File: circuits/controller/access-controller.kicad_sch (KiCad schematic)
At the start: 64 parts, among them J1 Conn_01x01_Female, J10 Terminal_01x03, J11 Terminal_01x04, J12 Screw_Terminal_01x05, J13 Conn_02x06_Odd_Even, J14 Terminal_01x04, J15 Terminal_01x03, J16 Terminal_01x03, J17 Terminal_01x03, J18 Terminal_01x04, J19 Screw_Terminal_01x05, J2 Conn_01x01_Female, J3 Conn_01x01_Female, J4 Conn_01x01_Female, J6 Screw_Terminal_01x02, J7 Terminal_01x04, J8 Terminal_01x03, J9 Barrel_Jack_Switch, J9 Terminal_01x03, Q3 Q_MMBT5551, U1 MCP23017_SS

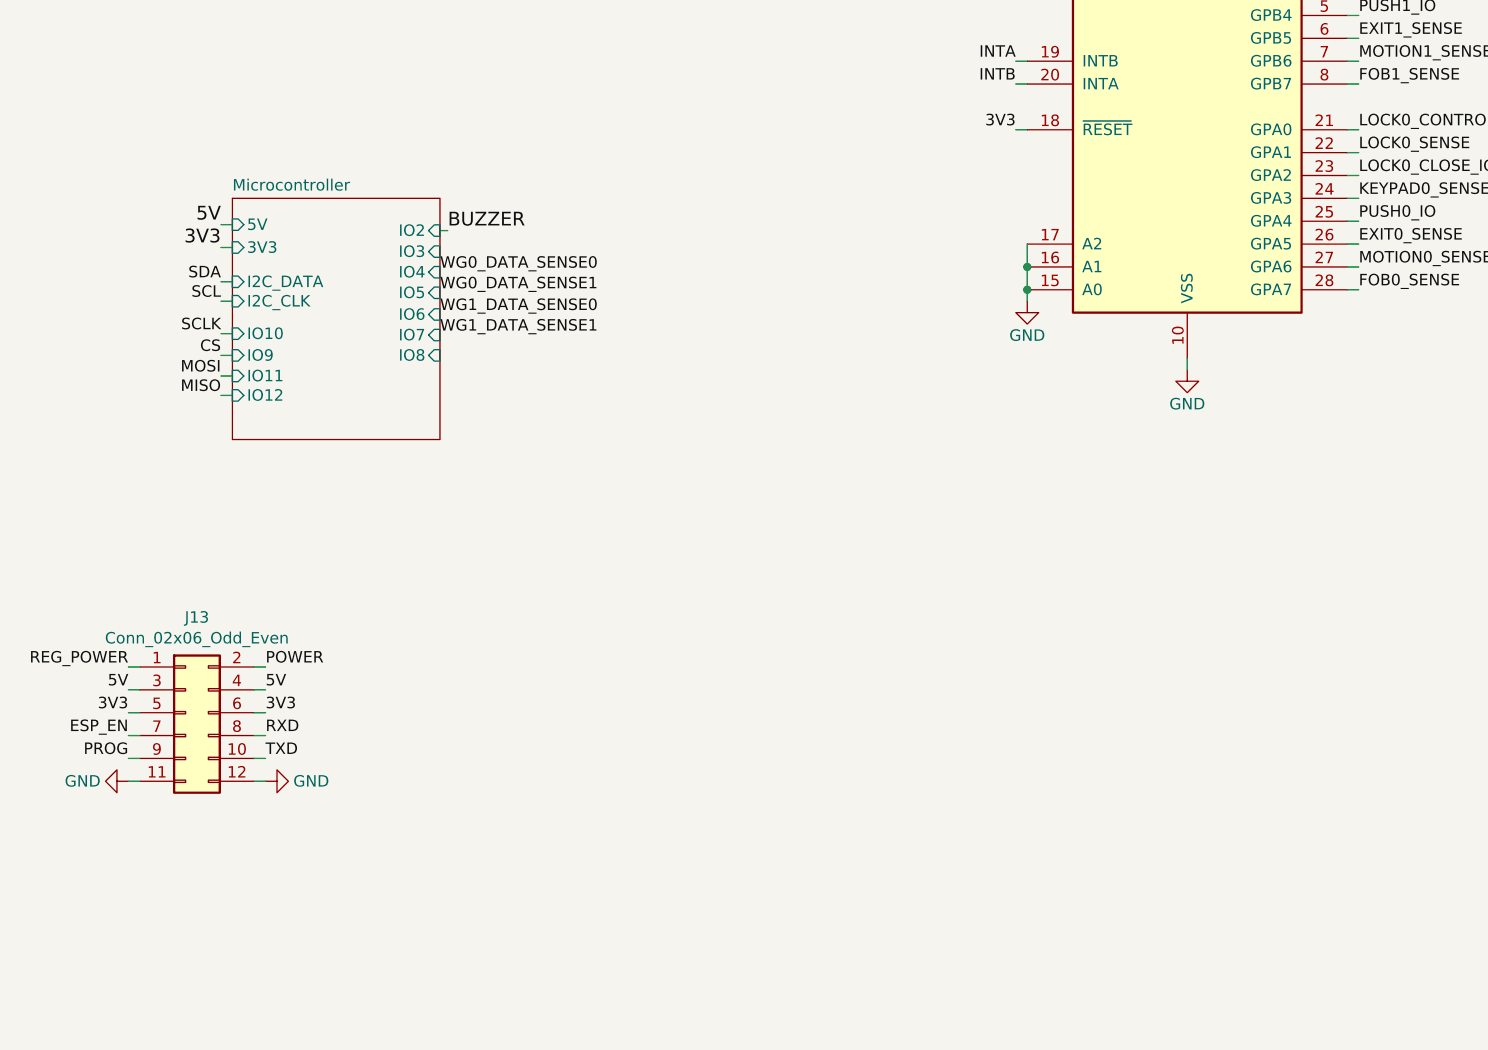
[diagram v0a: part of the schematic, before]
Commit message: order from fab
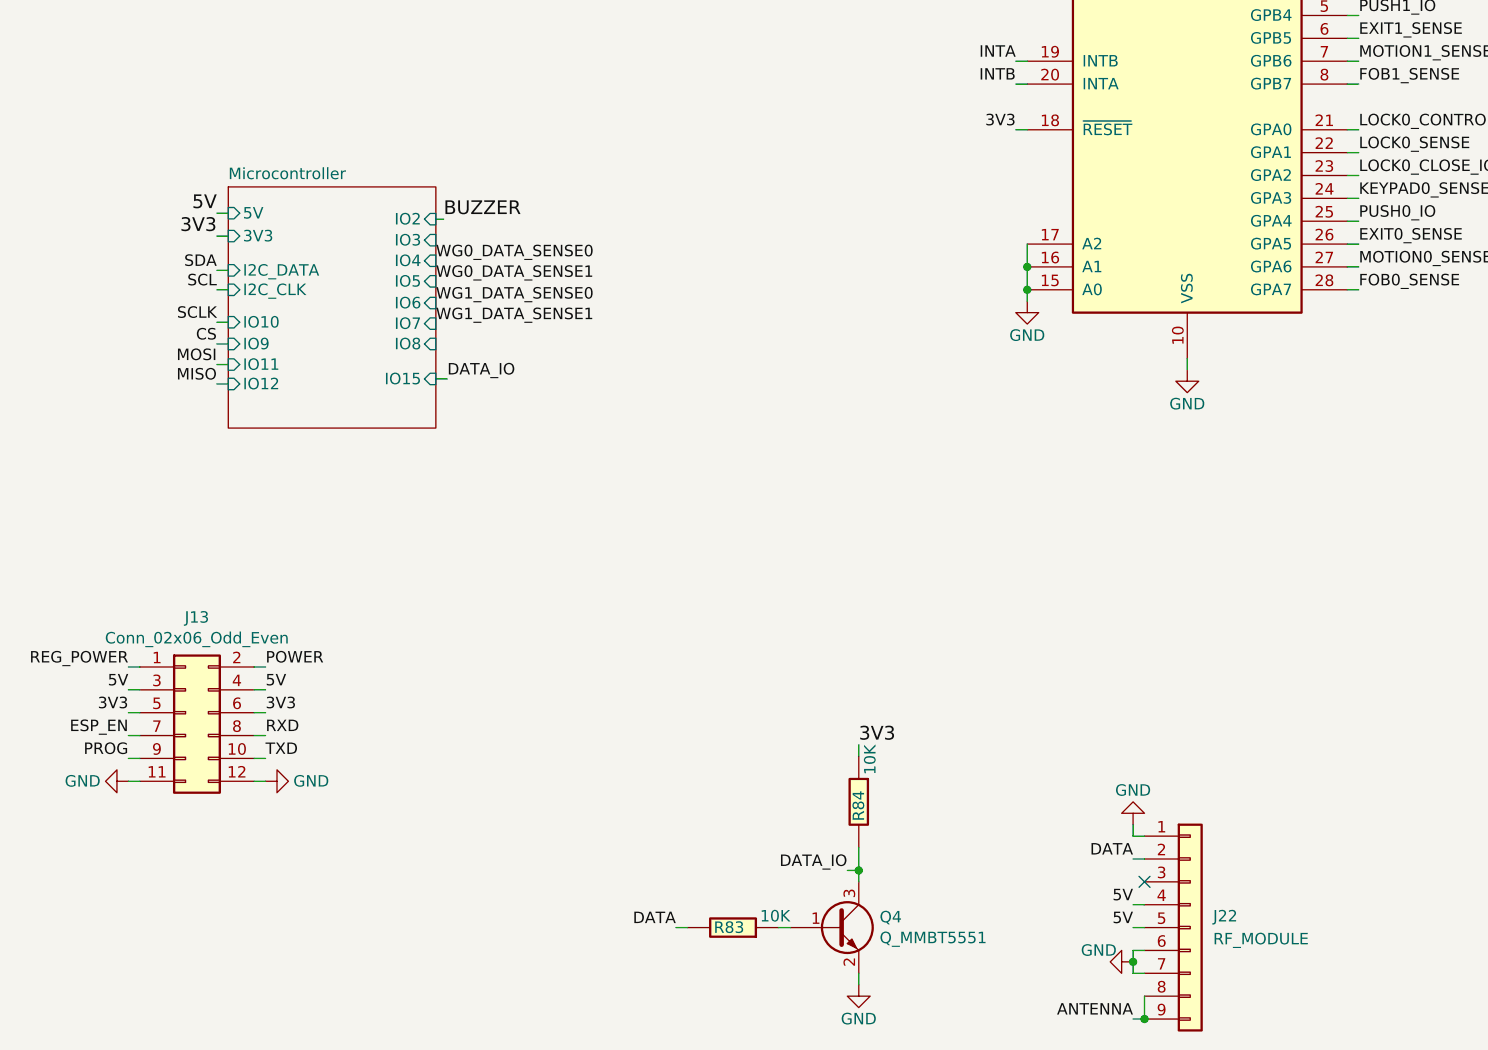
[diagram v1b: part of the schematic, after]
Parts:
- added J22: RF_MODULE, Library:RXB6_RF_MODULE, symbol Connector_Generic:Conn_01x09
- added Q4: Q_MMBT5551, Package_TO_SOT_SMD:SOT-23, symbol Open_Automation:Q_MMBT5551
- added R83, R84: 10K, Resistor_SMD:R_0402_1005Metric_Pad0.72x0.64mm_HandSolder, symbol Open_Automation:R_10K_0402
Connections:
- net 3V3: now also R84.1
- net 5V: now also J22.4 (Pin_4), J22.5 (Pin_5)
- net GND: now also J22.1 (Pin_1), J22.6 (Pin_6), J22.7 (Pin_7), Q4.2 (E)
- new net: Q4.1 (B), R83.1
- new net ANTENNA: J22.8 (Pin_8), J22.9 (Pin_9)
- new net DATA: J22.2 (Pin_2), R83.2
- new net DATA_IO: Q4.3 (C), R84.2
- no-connect marks 0 -> 1
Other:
- sheet Microcontroller ports: added IO15; removed none
